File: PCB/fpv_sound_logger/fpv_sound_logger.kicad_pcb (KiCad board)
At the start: 2 copper layers, 32.1 x 25.8 mm, 47 parts, among them CN1 SM04B-SRSS-TB(LF)(SN), IC1 W25Q128JVSIQ, IC2 NCP1117ST33T3G, J1 DM3D-SF, U1 RP2040, U2 INMP441ACEZ-R7, Y1 ABM8-272-T3

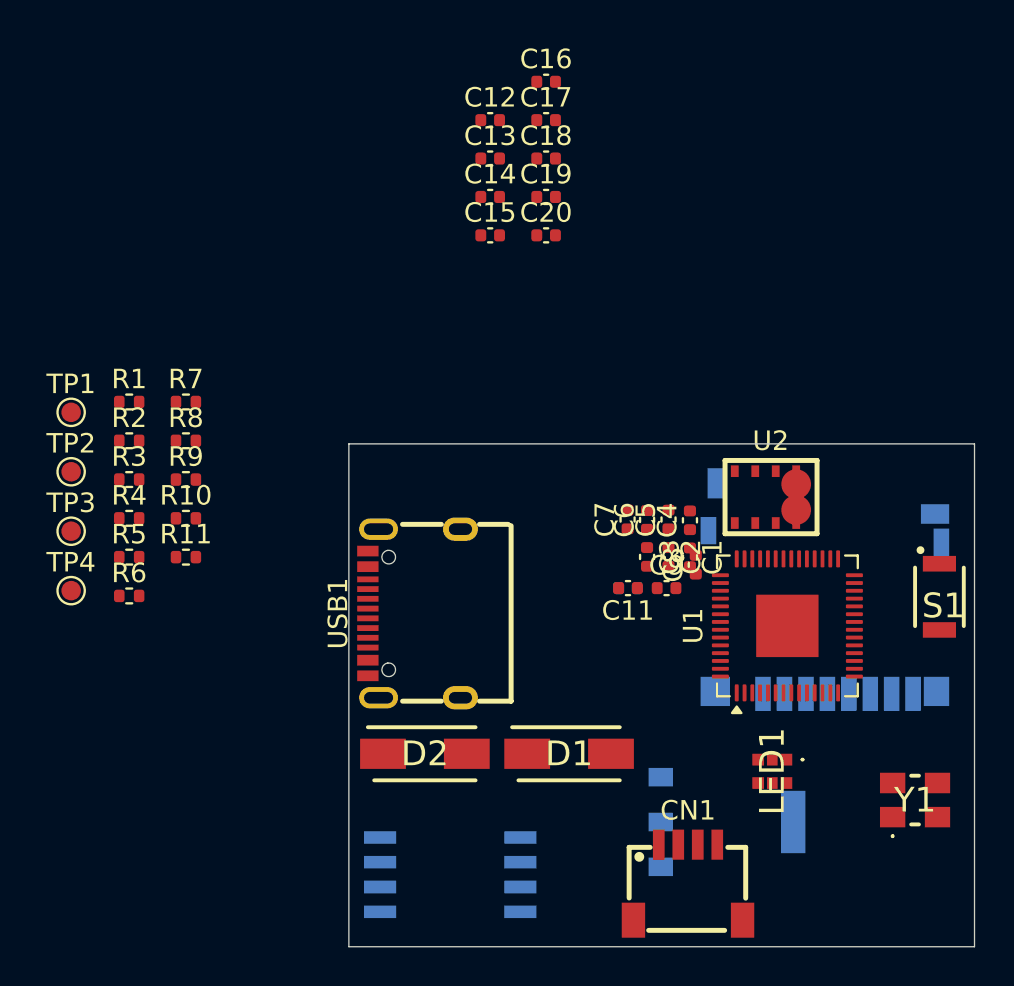
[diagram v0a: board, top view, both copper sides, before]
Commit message: PCB: started routing
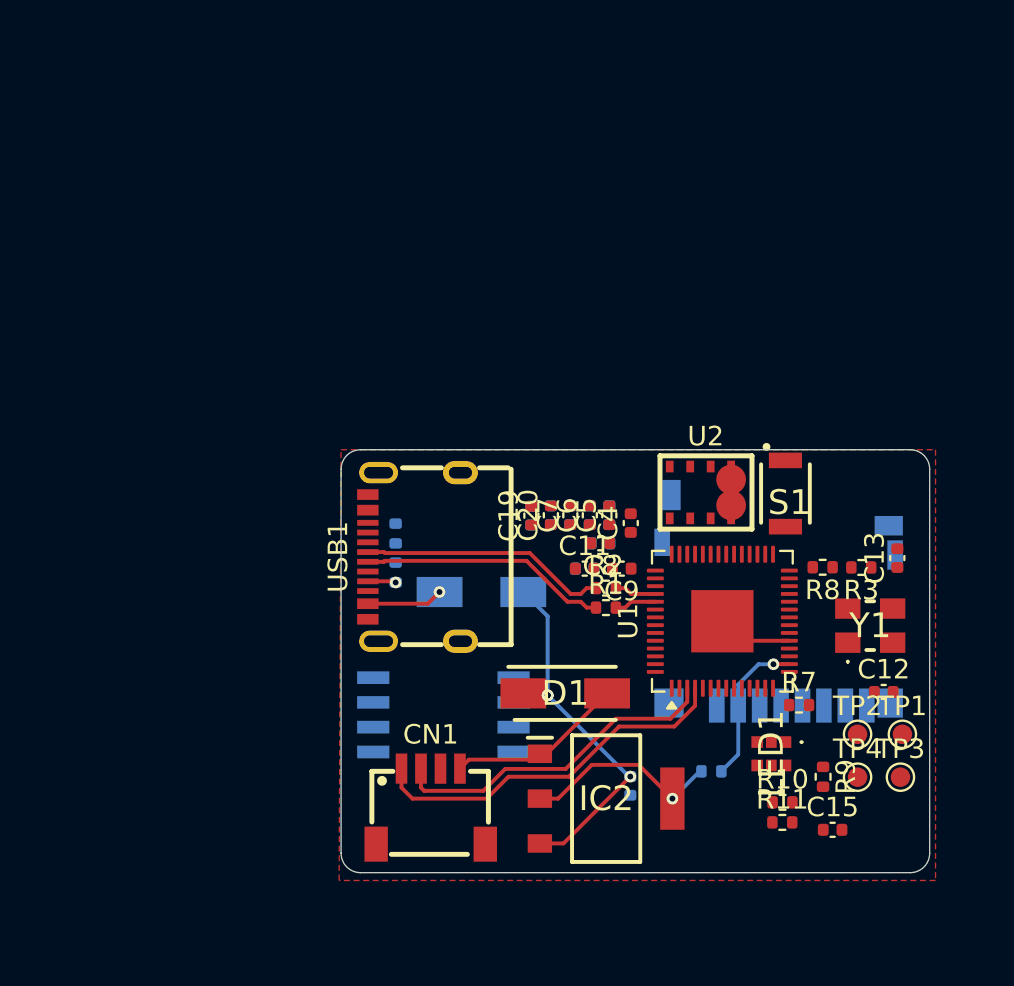
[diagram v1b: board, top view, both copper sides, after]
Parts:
- C1, C14, C16, C17, C18, C2, C3, D2, R4, R5, R6: moved to B.Cu
- IC2: moved to F.Cu
- moved TP1 45.7 mm to (152.8, 94.5)
- moved TP3 44.4 mm to (152.7, 96.7)
- moved TP2 42.5 mm to (150.5, 94.5)
- moved TP4 41.5 mm to (150.5, 96.7)
- moved R3 37.8 mm to (150.7, 85.9), turned to 180 degrees
- moved C16 36.4 mm to (138.8, 97.2), turned to -90 degrees
- moved R9 36.1 mm to (148.7, 96.7), turned to -90 degrees
- moved C12 35.6 mm to (151.8, 92.3)
- moved C15 35.2 mm to (149.2, 99.4)
- moved R7 35.1 mm to (147.5, 93.0)
- moved R10 33.9 mm to (146.7, 98.0)
- moved R11 33.5 mm to (146.6, 99.0)
- moved R8 33.3 mm to (148.7, 85.9), turned to 180 degrees
- moved R4 32.6 mm to (143.0, 96.4)
- moved C13 29.3 mm to (152.5, 85.5), turned to 90 degrees
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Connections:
- net Net-(U1-USB_DM) renamed /USB_DIFF-
- net Net-(U1-USB_DP) renamed /USB_DIFF+
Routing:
- net /GPIO2: track 0.00 -> 19.1 mm
- net VBUS: track 0.00 -> 19.1 mm, vias 0 -> 3
- net /GPIO1: track 0.00 -> 17.3 mm
- net /USB_D+: track 0.00 -> 12.7 mm
- net /USB_D-: track 0.00 -> 12.7 mm
- net +3V3: track 0.00 -> 10.3 mm, vias 0 -> 1
- net Net-(D1-A): track 0.00 -> 9.15 mm
- net /GPIO13: track 0.00 -> 7.87 mm, vias 0 -> 1
- net Net-(D2-K): track 0.00 -> 3.92 mm, vias 0 -> 1
- net GND: track 0.00 -> 3.85 mm
- net /USB_DIFF-: track 0.00 -> 2.15 mm
- net /USB_DIFF+: track 0.00 -> 2.15 mm
- net Net-(USB1-CC1): track 0.00 -> 1.45 mm, vias 0 -> 1
- added copper zone on F.Cu, net GND
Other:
- board size 32.1 x 25.8 mm -> 30.2 x 21.7 mm
